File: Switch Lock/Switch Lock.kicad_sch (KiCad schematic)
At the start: 6 parts, among them J1 Conn_01x06, SW1 SW_SPST, SW2 SW_SPST, SW3 SW_SPST, SW4 SW_SPST, SW5 SW_SPST

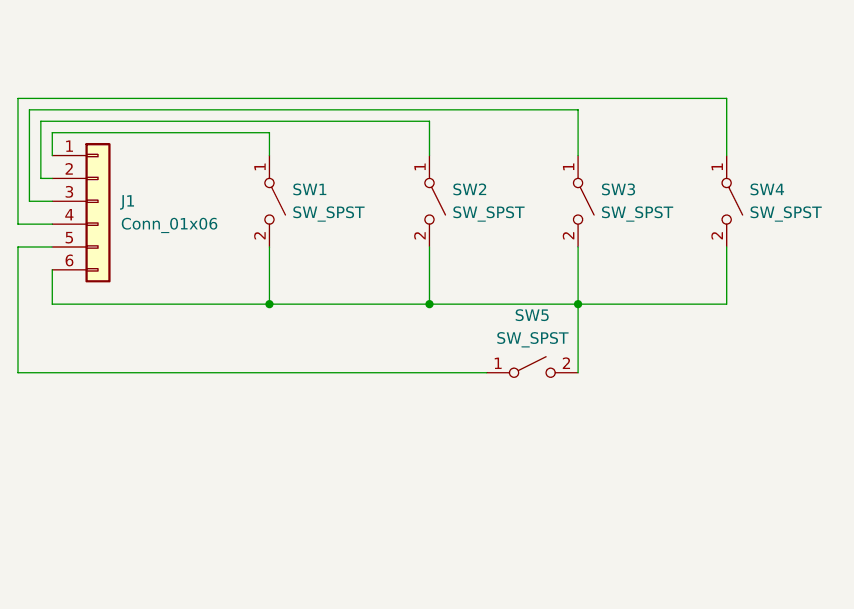
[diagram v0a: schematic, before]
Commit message: 123
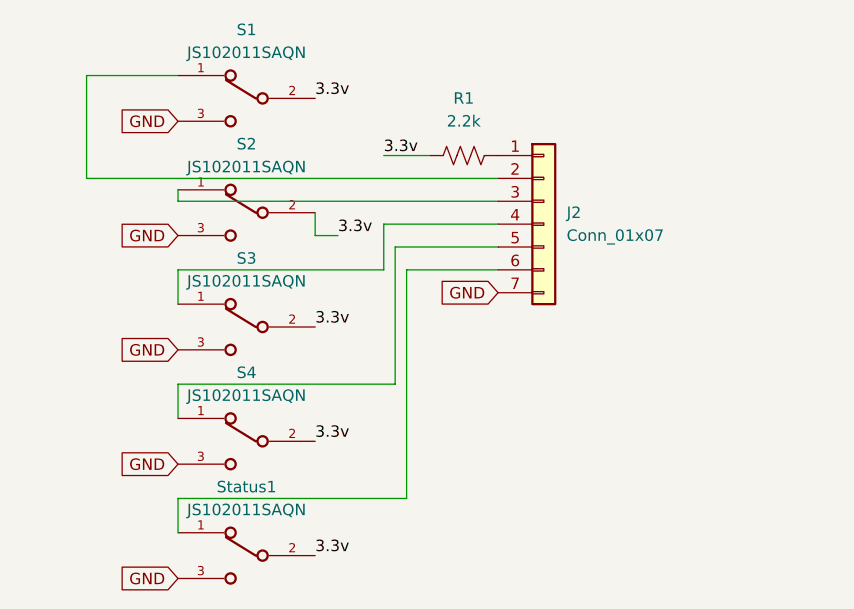
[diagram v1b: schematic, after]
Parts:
- removed J1: Conn_01x06, Connector_PinHeader_2.54mm:PinHeader_1x06_P2.54mm_Vertical, symbol Connector_Generic:Conn_01x06
- removed SW1, SW2, SW3, SW4, SW5: SW_SPST, symbol Switch:SW_SPST
- added J2: Conn_01x07, symbol Connector_Generic:Conn_01x07
- added R1: 2.2k, Resistor_SMD:R_0805_2012Metric_Pad1.20x1.40mm_HandSolder, symbol Device:R_US
- added S1, S2, S3, S4, Status1: JS102011SAQN, JS102011SAQN:SW_JS102011SAQN, symbol SS_js102011:JS102011SAQN
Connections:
- new net: J2.1 (Pin_1), R1.2
- new net: J2.5 (Pin_5), S4.1
- new net: J2.2 (Pin_2), S1.1
- new net: J2.3 (Pin_3), S2.1
- new net: J2.4 (Pin_4), S3.1
- new net: J2.6 (Pin_6), Status1.1
- new net 3.3v: R1.1, S1.2, S2.2, S3.2, S4.2, Status1.2
- new net GND: J2.7 (Pin_7), S1.3, S2.3, S3.3, S4.3, Status1.3

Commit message: finisheddesign
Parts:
- J2: footprint (none) -> Connector_PinHeader_2.54mm:PinHeader_1x07_P2.54mm_Vertical
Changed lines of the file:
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@@
 			)
 		)
-		(property "Footprint" ""
+		(property "Footprint" "Connector_PinHeader_2.54mm:PinHeader_1x07_P2.54mm_Vertical"
 			(at 104.14 66.04 0)
 			(effects
